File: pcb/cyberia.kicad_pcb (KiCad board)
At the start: 4 copper layers, 226.1 x 119.4 mm, 109 parts, among them J1 USB_C_Receptacle_USB2.0_16P, SW10 SW_Push, SW11 SW_Push, SW12 SW_Push, SW13 SW_Push, SW14 SW_Push, SW15 SW_Push, SW16 SW_Push, SW17 SW_Push, SW18 SW_Push, SW19 SW_Push, SW2 SW_Push, SW21 SW_Push, SW22 SW_Push, SW23 SW_Push, SW24 SW_Push, SW25 SW_Push, SW26 SW_Push, SW27 SW_Push, SW28 SW_Push, SW29 SW_Push, SW3 SW_Push, SW30 SW_Push, SW31 SW_Push, SW32 SW_Push, SW33 SW_Push, SW34 SW_Push, SW35 SW_Push, SW36 SW_Push, SW37 SW_Push, SW38 SW_Push, SW39 Reset, SW4 SW_Push, SW40 ROM, SW5 SW_Push, SW6 SW_Push, SW7 SW_Push, SW8 SW_Push, SW9 SW_Push, U1 RP2040, U2 AP2127N-3.3, U3 USBLC6-2SC6, U4 MX25R3235FZNxx0, Y1 Crystal_GND24

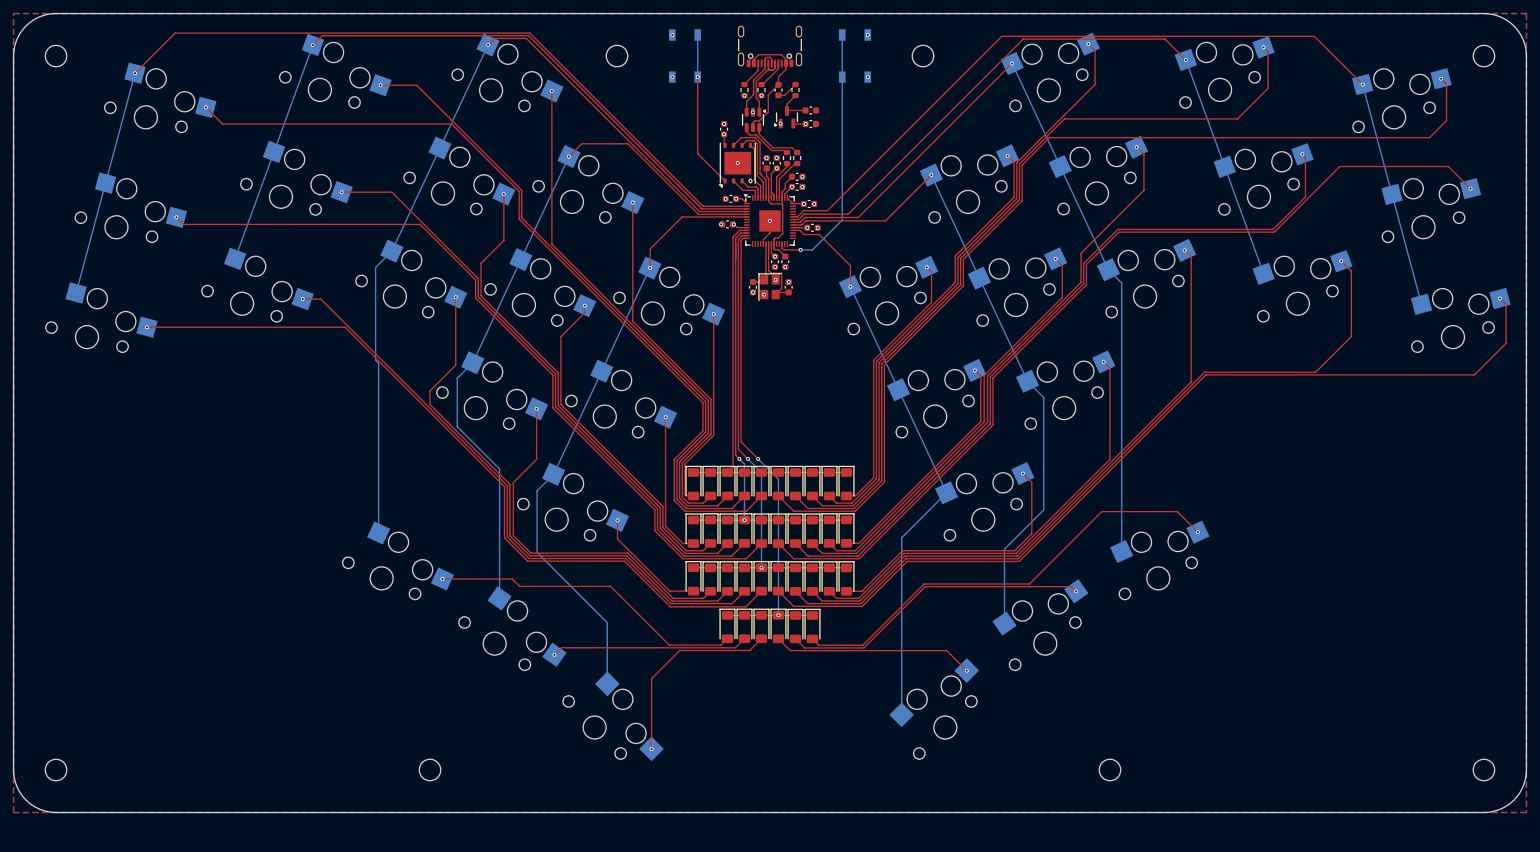
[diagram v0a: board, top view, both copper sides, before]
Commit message: rev.666
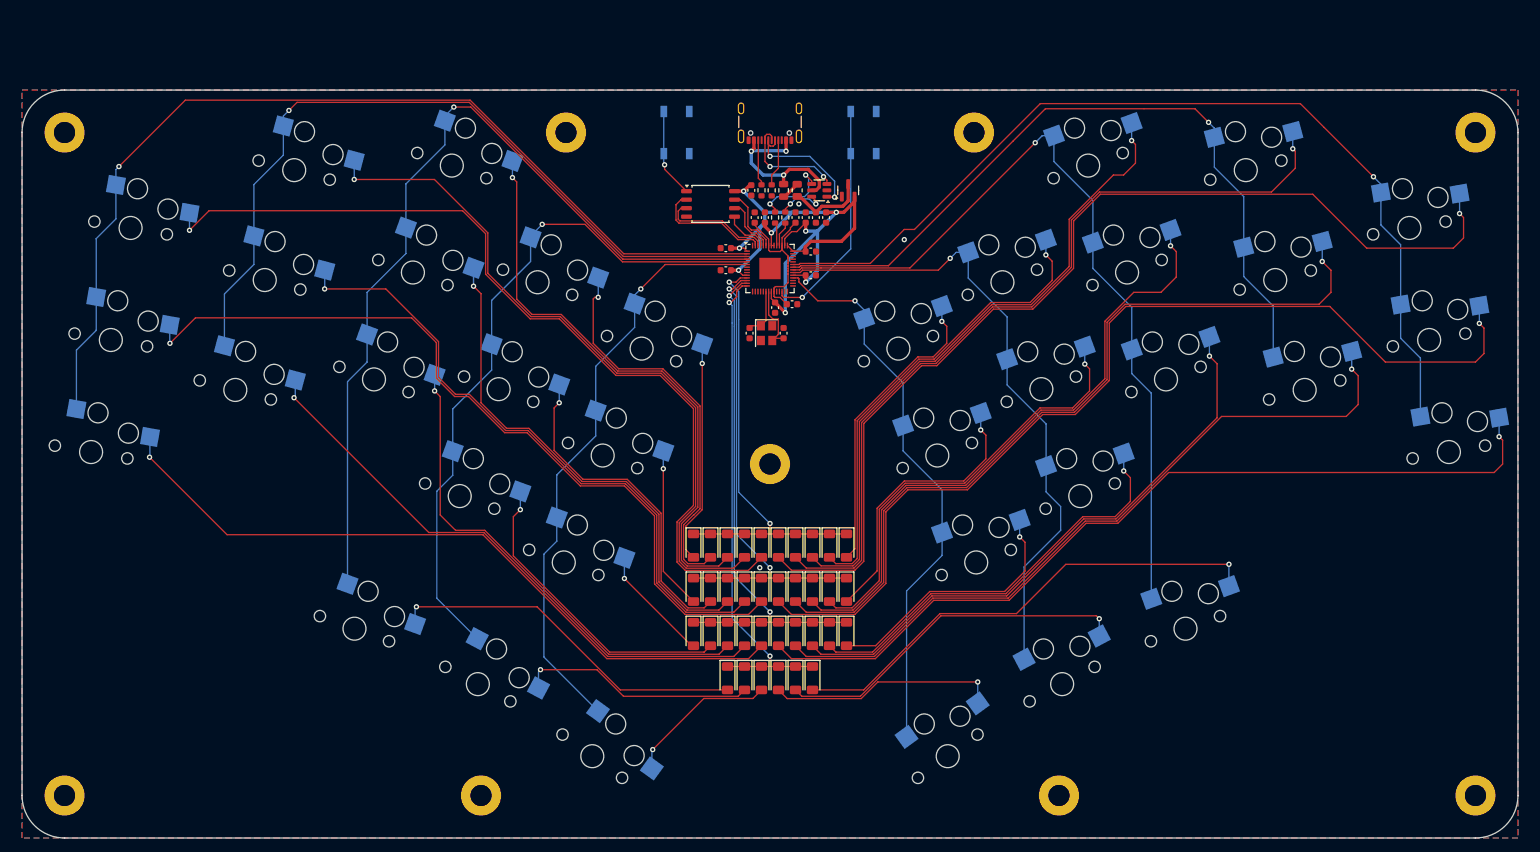
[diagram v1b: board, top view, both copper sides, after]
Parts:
- added H9: MountingHole_Pad, MountingHole:MountingHole_3.2mm_M3, F.Cu at (203.2, 128.3)
- F1: footprint Fuse:Fuse_0603_1608Metric -> Fuse:Fuse_0805_2012Metric
- FB1: footprint Resistor_SMD:R_0603_1608Metric -> Resistor_SMD:R_0805_2012Metric
- SW10, SW11, SW12, SW13, SW14, SW15, SW16, SW17, SW18, SW19, SW2, SW21, SW22, SW23, SW24, SW25, SW26, SW27, SW28, SW29, SW3, SW30, SW31, SW32, SW33, SW34, SW35, SW36, SW37, SW38, SW4, SW5, SW6, SW7, SW8, SW9: value SW_Push -> (none)
- U4: value MX25R3235FZNxx0 -> W25Q128JVSIQ; footprint Package_SON:WSON-8-1EP_6x5mm_P1.27mm_EP3.4x4mm -> Package_SO:SOIC-8_5.3x5.3mm_P1.27mm
- moved H4 232.5 mm to (308.6, 78.7)
- moved H5 137.9 mm to (97.8, 177.8)
- moved H2 137.6 mm to (172.7, 78.7)
- moved H6 128.7 mm to (160.0, 177.8)
- moved H3 122.0 mm to (233.7, 78.7)
- moved H7 94.1 mm to (246.4, 177.8)
- moved H8 54.7 mm to (308.6, 177.8)
- moved SW21 17.2 mm to (304.6, 126.5), turned to 10 degrees
- moved SW2 17.2 mm to (101.8, 126.5), turned to -10 degrees
- moved SW3 16.9 mm to (104.7, 109.7), turned to -10 degrees
- moved SW22 16.9 mm to (301.7, 109.7), turned to 10 degrees
- moved SW4 16.7 mm to (107.7, 93.0), turned to -10 degrees
- moved SW23 16.7 mm to (298.7, 93.0), turned to 10 degrees
- moved C8 16.0 mm to (210.1, 91.4), turned to -90 degrees
- moved R3 15.2 mm to (201.9, 87.4)
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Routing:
- net +3.3V: track 22.9 -> 112.7 mm, vias 9 -> 8
- net SD1: track 4.91 -> 17.9 mm
- net SD2: track 4.25 -> 16.6 mm
- net Net-(D22-A): track 135.9 -> 148.0 mm
- net Net-(U4-~{CS}): track 23.5 -> 13.3 mm
- net D-: track 10.3 -> 20.2 mm, vias 0 -> 2
- net Net-(D11-A): track 54.2 -> 45.9 mm
- net Net-(D25-A): track 111.6 -> 119.9 mm
- net Net-(D7-A): track 98.4 -> 106.5 mm
- net Net-(D28-A): track 86.1 -> 94.2 mm
- net C0: track 138.6 -> 146.3 mm
- net VBUS: track 18.6 -> 26.1 mm, vias 0 -> 3
- net C1: track 110.1 -> 117.6 mm
- net Net-(D17-A): track 47.1 -> 54.3 mm
- net Net-(D37-A): track 46.6 -> 53.6 mm
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- removed copper zone on In1.Cu, net +3.3V
- removed copper zone on In2.Cu, net GND
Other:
- board size 226.1 x 119.4 mm -> 223.5 x 111.8 mm
- copper layers 4 -> 2
